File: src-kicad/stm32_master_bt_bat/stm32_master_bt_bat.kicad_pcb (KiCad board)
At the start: 2 copper layers, 50 x 50 mm, 31 parts, among them J1 Conn_01x02_Male, J2 Conn_01x02_Male, J3 Conn_02x04_Odd_Even, J4 Conn_01x06_Female, Q1 Si2371EDS, SW1 SW_Push, SW2 SW_DIP_x01, U1 STM32F031F6Px, Y1 8M

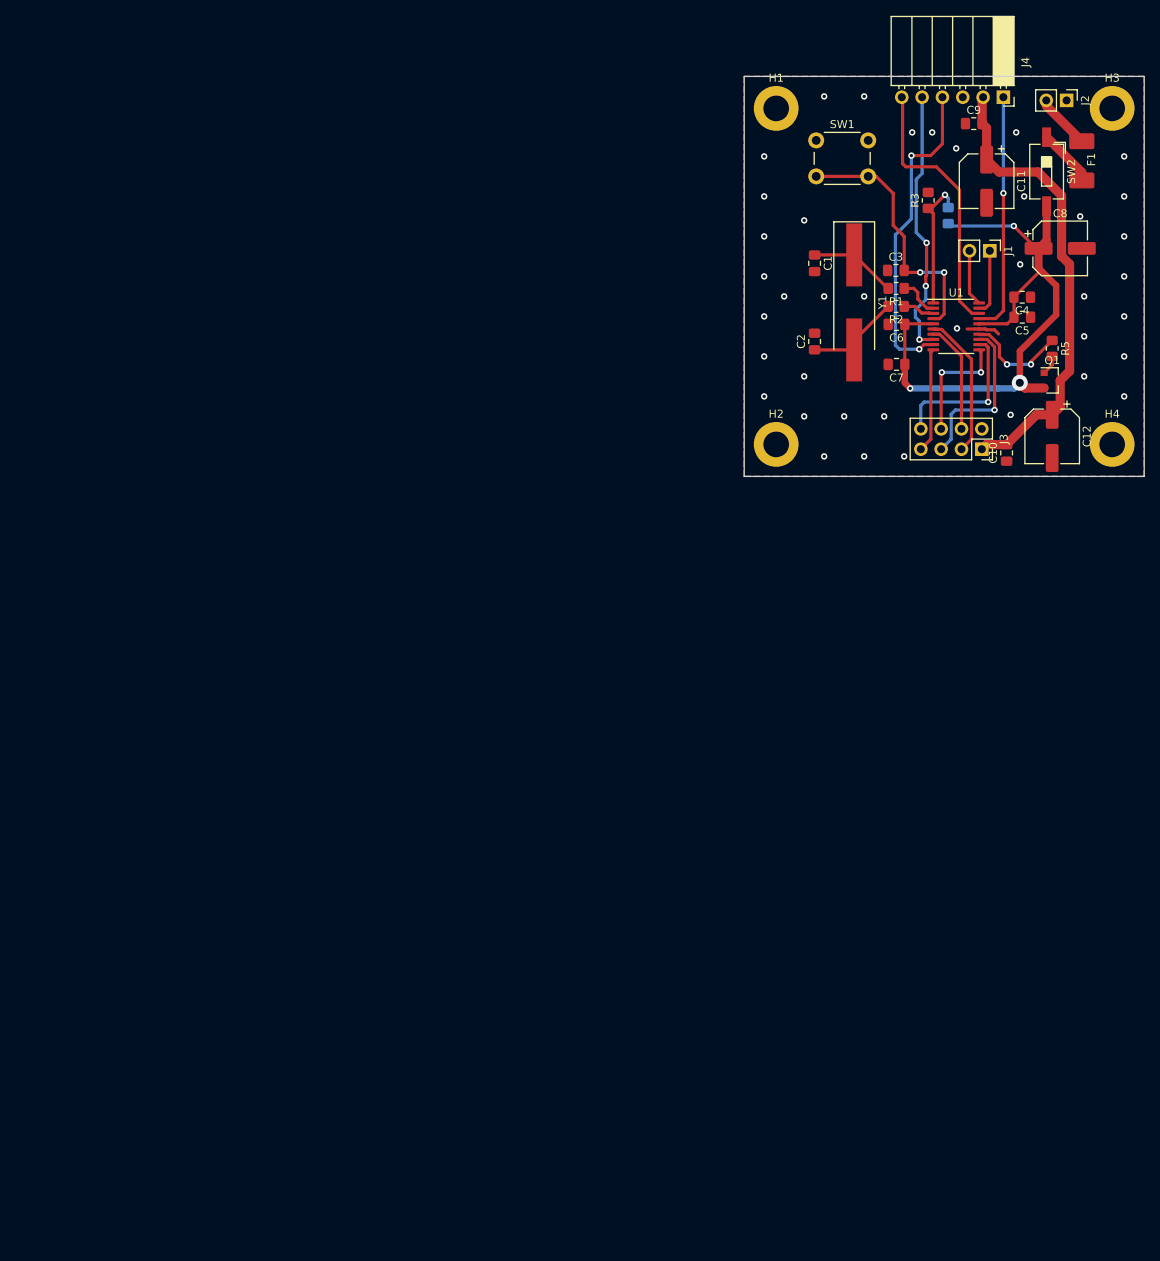
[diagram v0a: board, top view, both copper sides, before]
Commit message: update src-kicad directory (all files)
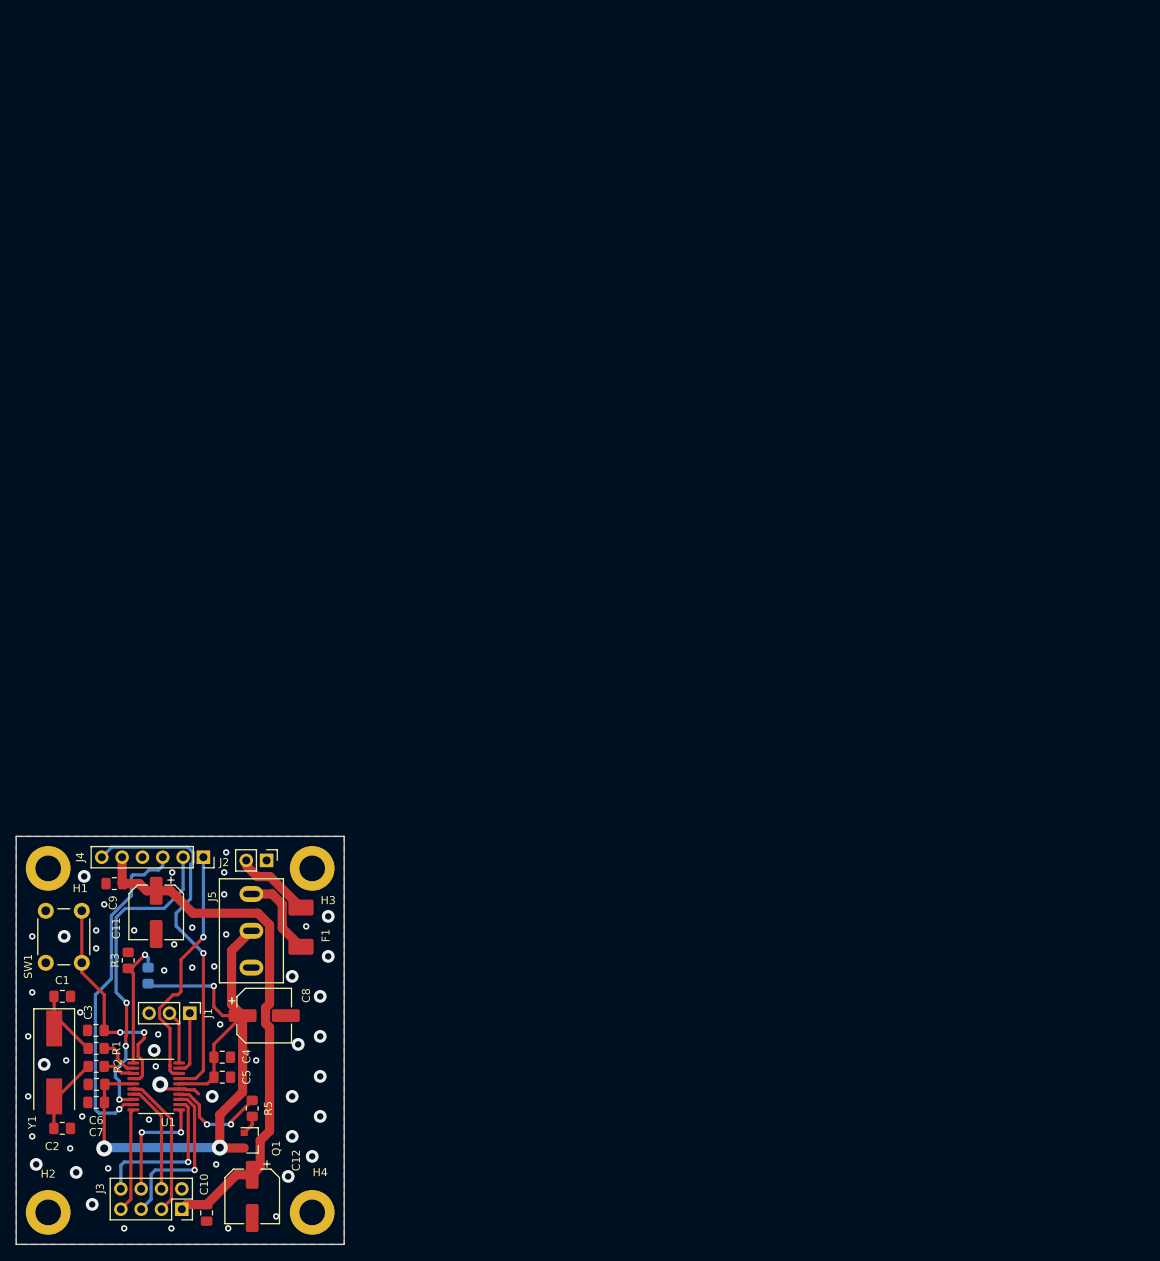
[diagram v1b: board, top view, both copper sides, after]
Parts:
- removed SW2: SW_DIP_x01, Button_Switch_SMD:SW_DIP_SPSTx01_Slide_6.7x4.1mm_W8.61mm_P2.54mm_LowProfile
- added J5: Conn_01x03, przelbl1x3:PRZELBL1X3, F.Cu at (133.4, 206.8)
- J1: value Conn_01x02_Male -> Conn_01x03_Male; footprint Connector_PinHeader_2.54mm:PinHeader_1x02_P2.54mm_Vertical -> Connector_PinHeader_2.54mm:PinHeader_1x03_P2.54mm_Vertical
- J4: footprint Connector_PinSocket_2.54mm:PinSocket_1x06_P2.54mm_Horizontal -> Connector_PinSocket_2.54mm:PinSocket_1x06_P2.54mm_Vertical
- Y1: footprint Crystal:Crystal_SMD_HC49-SD_HandSoldering -> Crystal:Crystal_SMD_HC49-SD
- moved C9 143.4 mm to (116.3, 200.9)
- moved SW1 140.9 mm to (107.7, 210.8), turned to 90 degrees
- moved C11 138.3 mm to (121.5, 204.5)
- moved C8 138.2 mm to (135.0, 217.4)
- moved J1 138.1 mm to (125.7, 217.1)
- moved C10 137.9 mm to (127.8, 242.1)
- moved C12 137.9 mm to (133.5, 240.0)
- moved C3 137.9 mm to (114.0, 219.2)
- moved C4 137.9 mm to (129.8, 222.6)
- moved C5 137.9 mm to (129.8, 225.1)
- moved C6 137.9 mm to (114.0, 226.0)
- moved H3 137.9 mm to (141.0, 199.0)
- moved H4 137.9 mm to (141.0, 241.0)
- moved J2 137.9 mm to (135.3, 198.0)
- moved J3 137.9 mm to (124.7, 241.6)
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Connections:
- J4 pad 1: HM-10_STATE -> HM-10-BRK
- J4 pad 2: Vcc -> UART1_TXD
- J4 pad 3: GND -> UART1_RXD
- J4 pad 4: UART1_RXD -> GND
- J4 pad 5: UART1_TXD -> Vcc
- J4 pad 6: HM-10-BRK -> HM-10_STATE
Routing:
- net HM-10_STATE: track 30.1 -> 45.2 mm
- net Vcc: track 59.1 -> 67.7 mm
- net +3V3: track 81.7 -> 88.0 mm
- net UART1_TXD: track 33.7 -> 39.7 mm
- net Net-(C3-Pad2): track 32.6 -> 28.5 mm
- net Net-(F1-Pad2): track 7.23 -> 10.7 mm
- net HM-10-BRK: track 33.8 -> 31.1 mm, vias 0 -> 1
- net Net-(F1-Pad1): track 6.94 -> 9.01 mm
- net UART1_RXD: track 40.0 -> 41.9 mm, vias 2 -> 1
- net Net-(C1-Pad1): track 10.9 -> 9.99 mm
- net Net-(C2-Pad1): track 12.2 -> 11.2 mm
- net GND: vias 39 -> 56
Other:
- board size 50 x 50 mm -> 41 x 51 mm
